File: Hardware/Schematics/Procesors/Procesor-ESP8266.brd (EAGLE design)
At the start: 35.5 x 37.8 mm, 7 parts

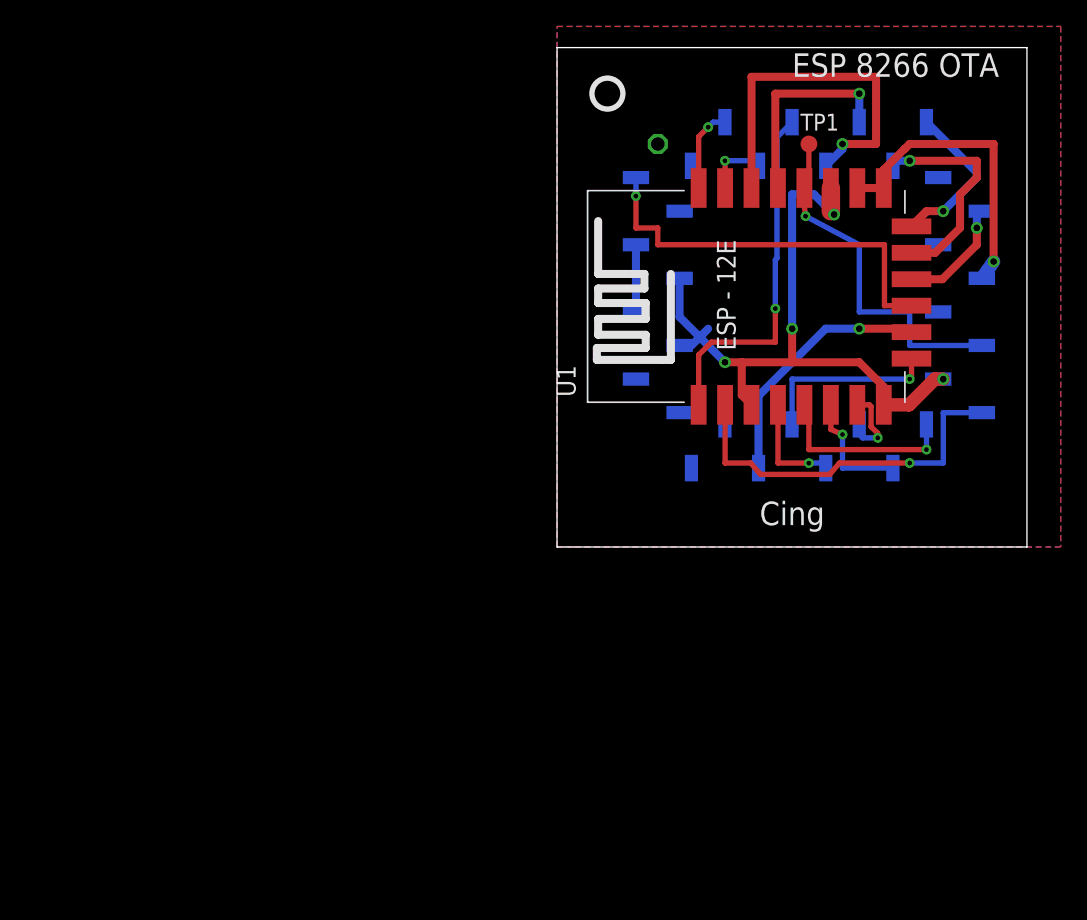
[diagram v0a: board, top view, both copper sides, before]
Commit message: commit
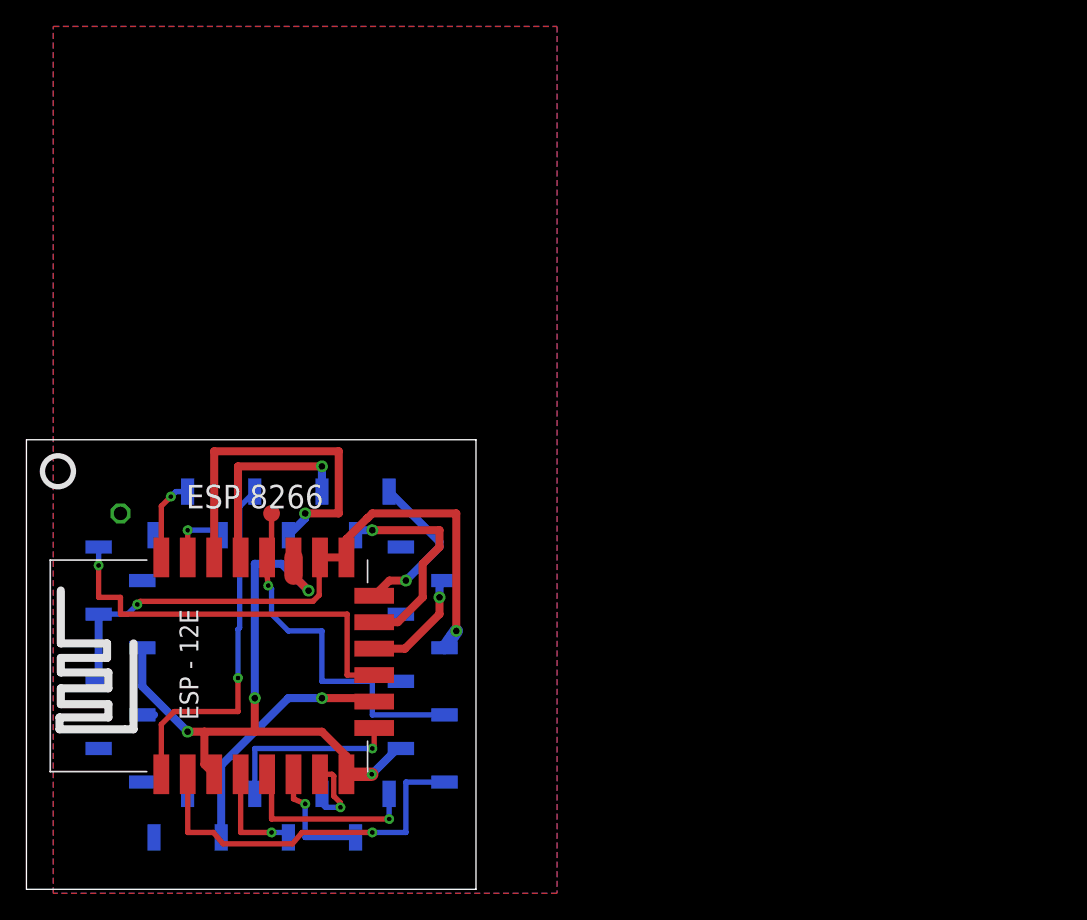
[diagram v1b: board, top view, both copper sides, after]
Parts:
- moved J3 49.3 mm to (-6.35, -11.4)
- moved J4 49.3 mm to (14.0, -8.89)
- moved U1 49.3 mm to (0.00, 0.00)
- moved J1 49.3 mm to (11.4, 11.4)
- moved J2 49.3 mm to (-8.89, 8.89)
- moved JP5 49.3 mm to (-8.89, 11.4)
- moved TP1 49.3 mm to (2.54, 11.4)
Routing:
- net GND: track 28.0 -> 48.2 mm, vias 1 -> 2
- net A2: track 15.3 -> 12.2 mm
- net A5: track 27.6 -> 26.9 mm
- net A6: track 27.1 -> 27.8 mm
- net +5V: track 52.4 -> 51.8 mm
- net A4: track 15.7 -> 15.2 mm
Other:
- board size 35.5 x 37.8 mm -> 34 x 34 mm
- board text added: "ESP 8266"
- board text removed: "Cing"
- board text removed: "ESP 8266 OTA"
